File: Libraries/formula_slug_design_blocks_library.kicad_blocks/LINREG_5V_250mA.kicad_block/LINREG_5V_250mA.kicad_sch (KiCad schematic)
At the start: 3 parts

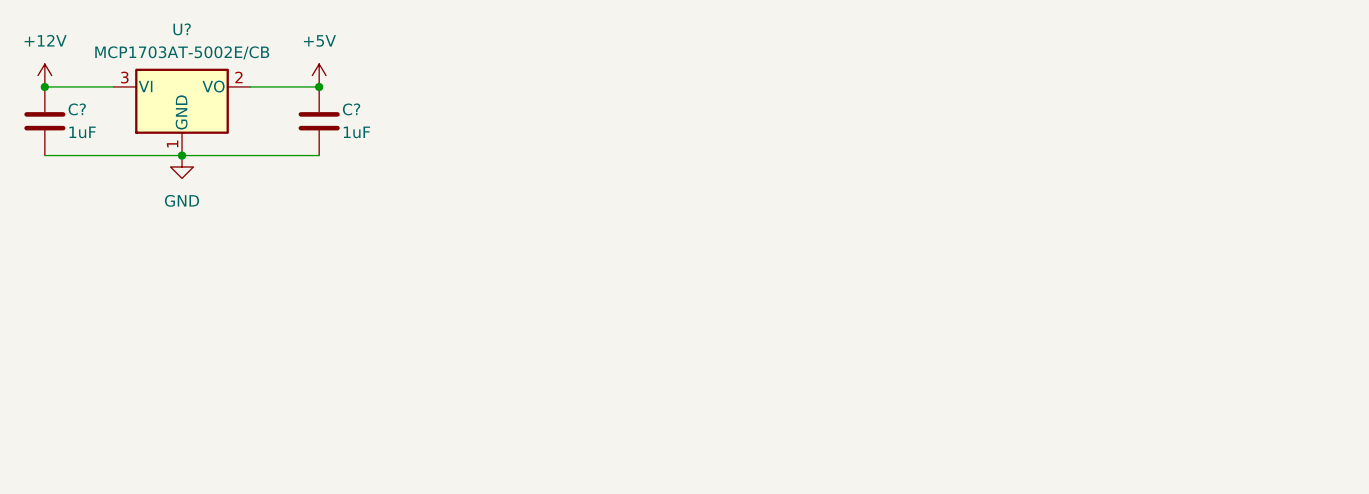
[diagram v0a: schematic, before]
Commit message: Fixed cap digi url links
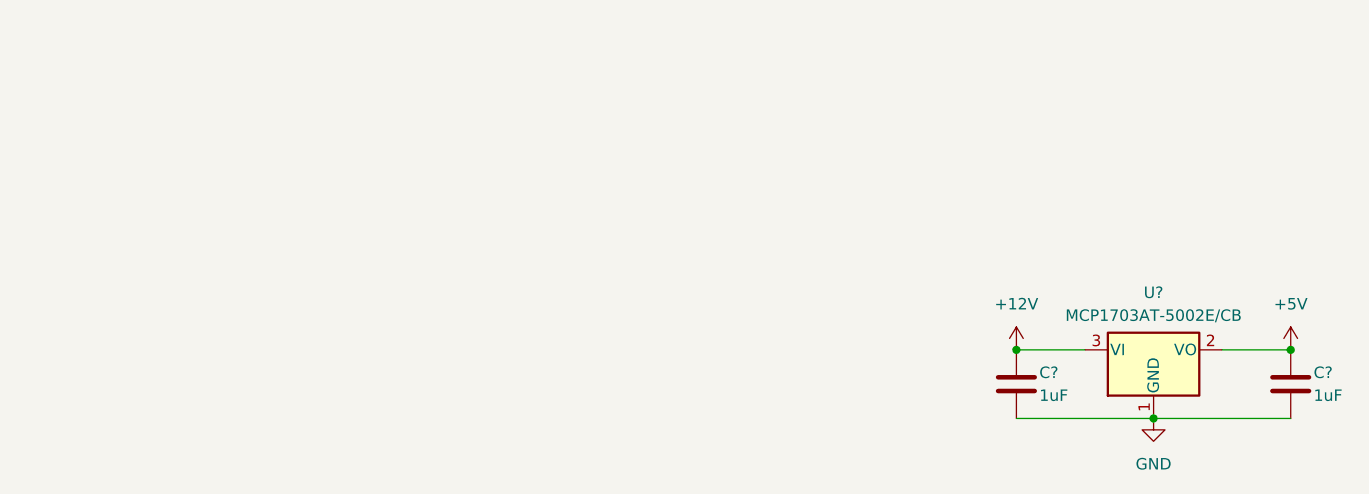
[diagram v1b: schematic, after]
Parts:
- C? (x2): Digi URL (none) -> https://www.digikey.com/en/products/detail/samsung-electro-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
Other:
- moved on the sheet: C?, U?
